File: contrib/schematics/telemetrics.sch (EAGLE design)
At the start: 26 parts, among them IC1 ATMEGA644-20PU, IC3 MAX232, IC4 MAX3232CPE, Q1 10Mhz

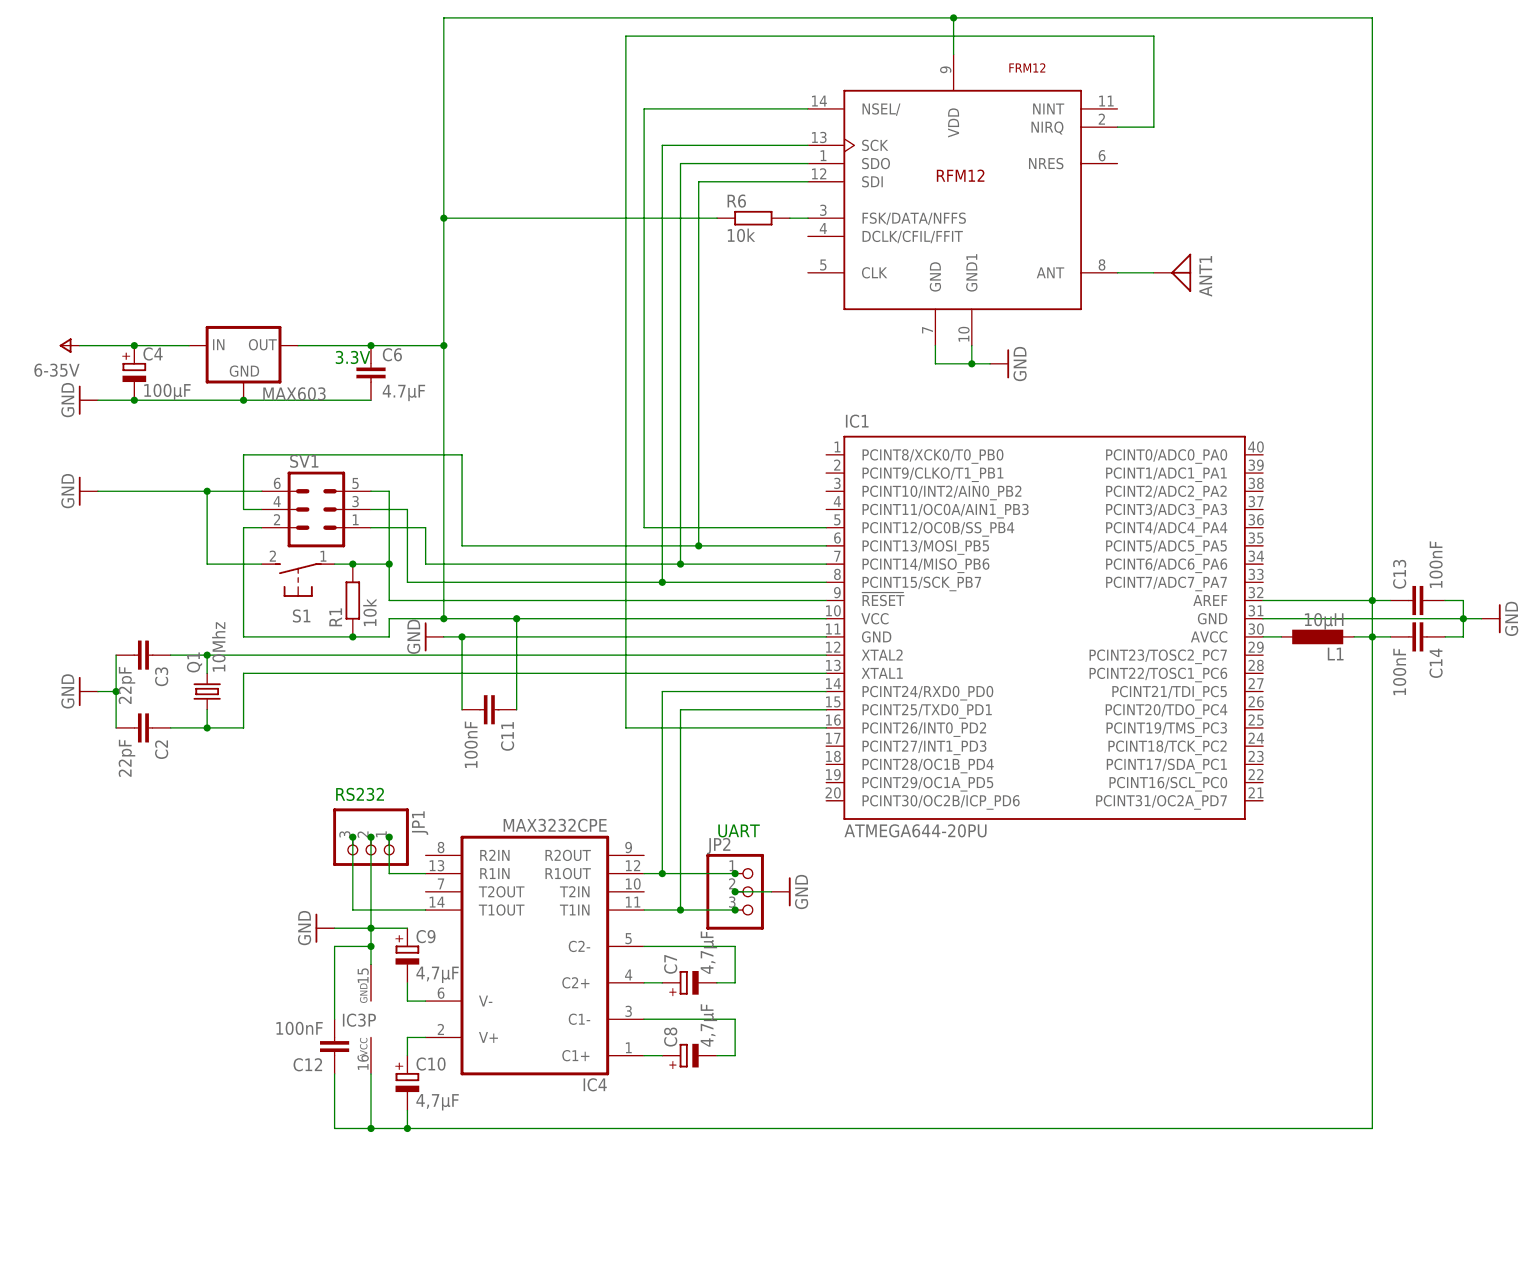
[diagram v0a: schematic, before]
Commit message: Updated telemetrics board
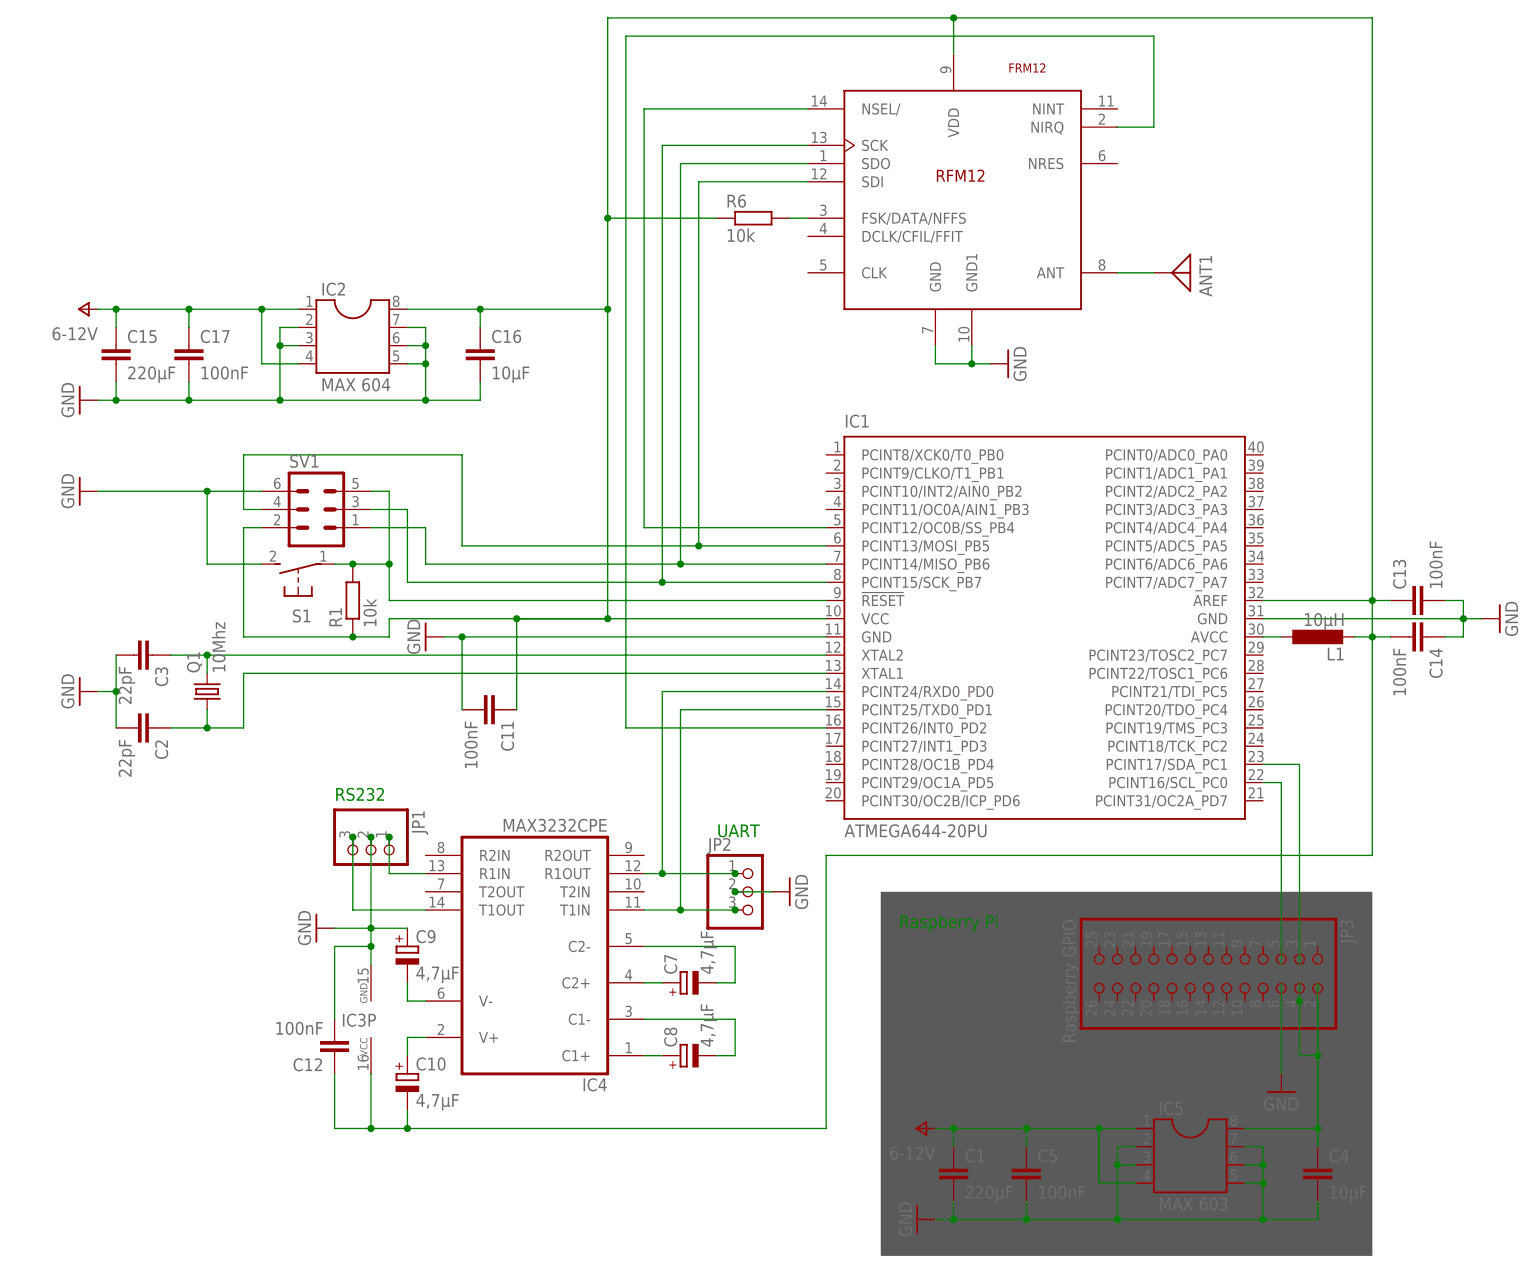
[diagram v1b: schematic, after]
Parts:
- removed C6: 4.7µF, capacitor-wima:C2.5/6
- removed MAX603: (no value), v-reg:78XXL
- added C1, C15: 220µF, capacitor-wima:C2.5/6
- added C16: 10µF, capacitor-wima:C2.5/5
- added C17, C5: 100nF, capacitor-wima:C2.5/2
- added IC2: MAX 604, ic-package:DIL8S
- added IC5: MAX 603, ic-package:DIL8S
- added JP3: Raspberry GPIO, pinhead:PINHD-2X13
- C4: value 100µF -> 10µF; device rcl:CPOL-EUE5-6 -> capacitor-wima:C2.5/5
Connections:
- new net N$21: IC1.PCINT17/SDA_PC1, JP3.3
- new net N$22: IC1.PCINT16/SCL_PC0, JP3.5
- new net VDD1: C4.1, IC5.8, JP3.2, JP3.4
- net GND: now also C1.2, C15.2, C16.2, C17.2, C4.2, C5.2, IC2.2, IC2.3, IC2.5, IC2.6, IC2.7, IC5.2, IC5.3, IC5.5, IC5.6, IC5.7, JP3.6; no longer C4.-, C6.2, MAX603.GND
- net V+: now also C1.1, C15.1, C17.1, C5.1, IC2.1, IC2.4, IC5.1, IC5.4; no longer C4.+, MAX603.IN
- net VDD: now also C16.1, IC2.8; no longer C6.1, MAX603.OUT
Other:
- note added: "Raspberry PI"
- note removed: "3.3V"
